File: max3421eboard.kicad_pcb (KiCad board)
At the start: 2 copper layers, 41 x 49 mm, 32 parts, among them J1 USB A, J2 USB MicroB, J3 1x10, J4 1x8, J5 1x8, J6 1x3, J7 Conn_01x04, U1 MAX3421E, U2 LP2985-3.3, U3 STMPS2141STR, Y1 12MHz

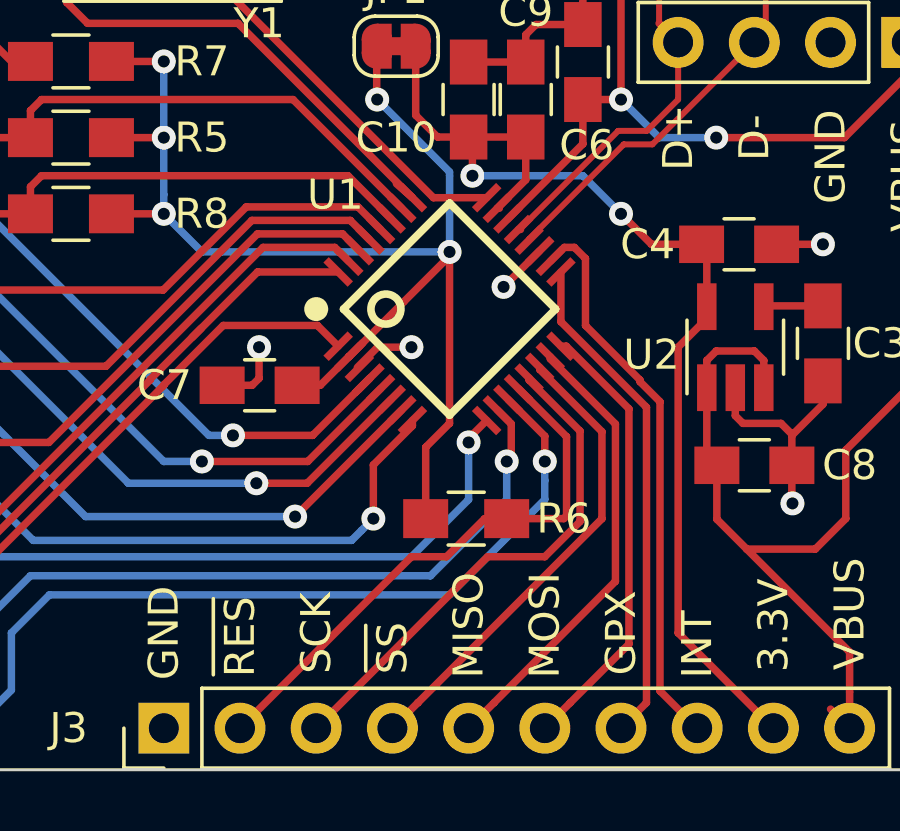
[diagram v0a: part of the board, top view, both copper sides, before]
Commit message: Fix the board layout
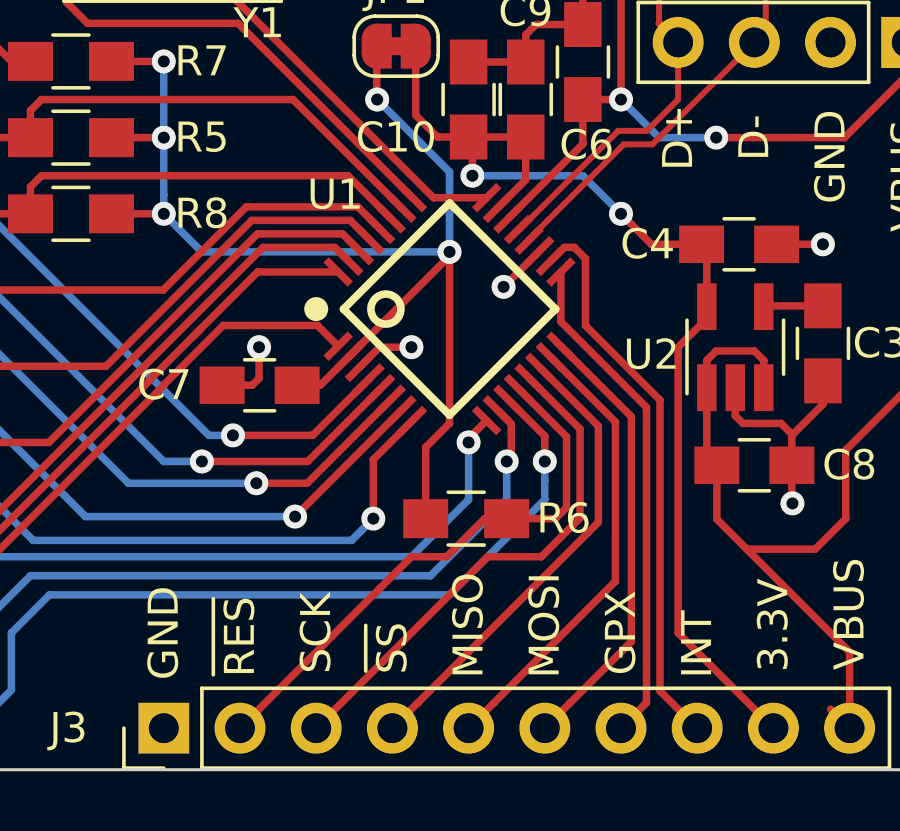
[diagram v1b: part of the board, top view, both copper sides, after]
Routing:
- net /X+: track 21.4 -> 20.7 mm
